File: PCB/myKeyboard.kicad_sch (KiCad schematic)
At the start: 6 parts, among them SW1 SW_Push, SW2 SW_Push, SW3 SW_Push, U1 XIAO-RP2040-DIP

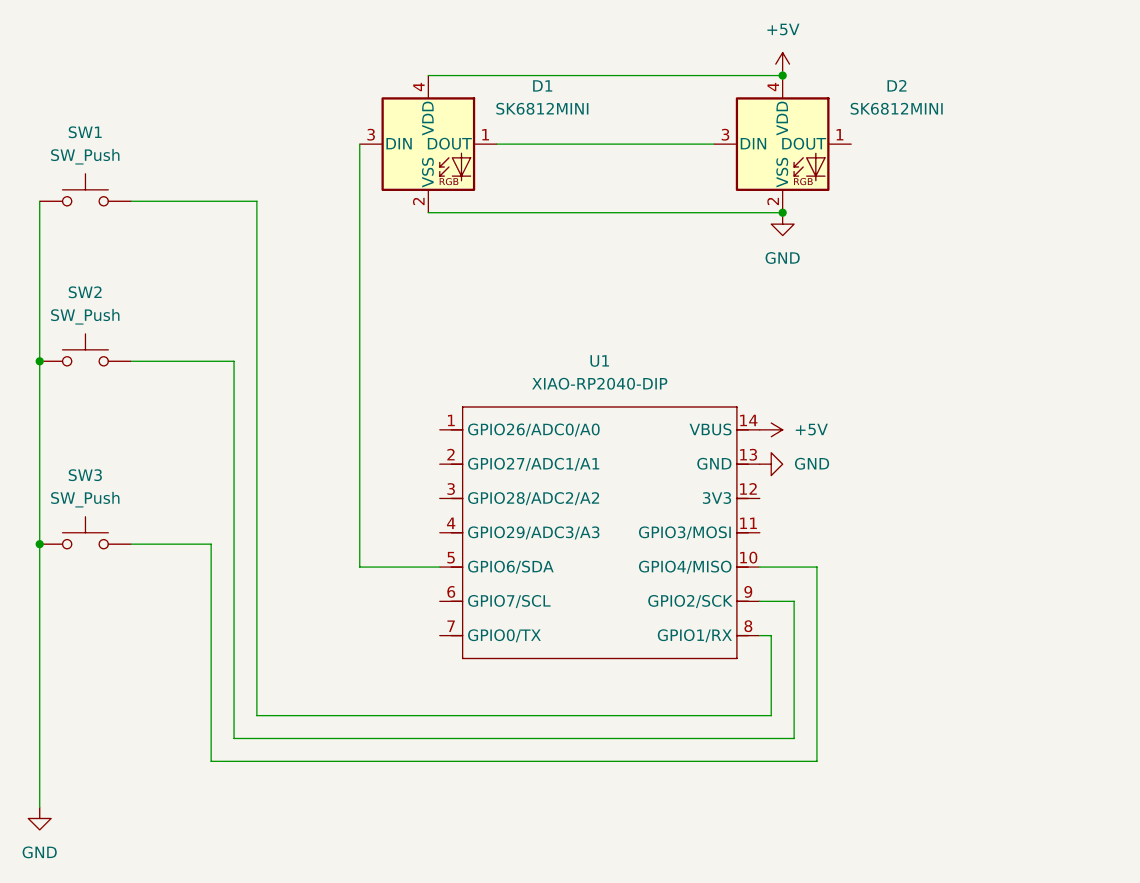
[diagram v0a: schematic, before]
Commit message: a
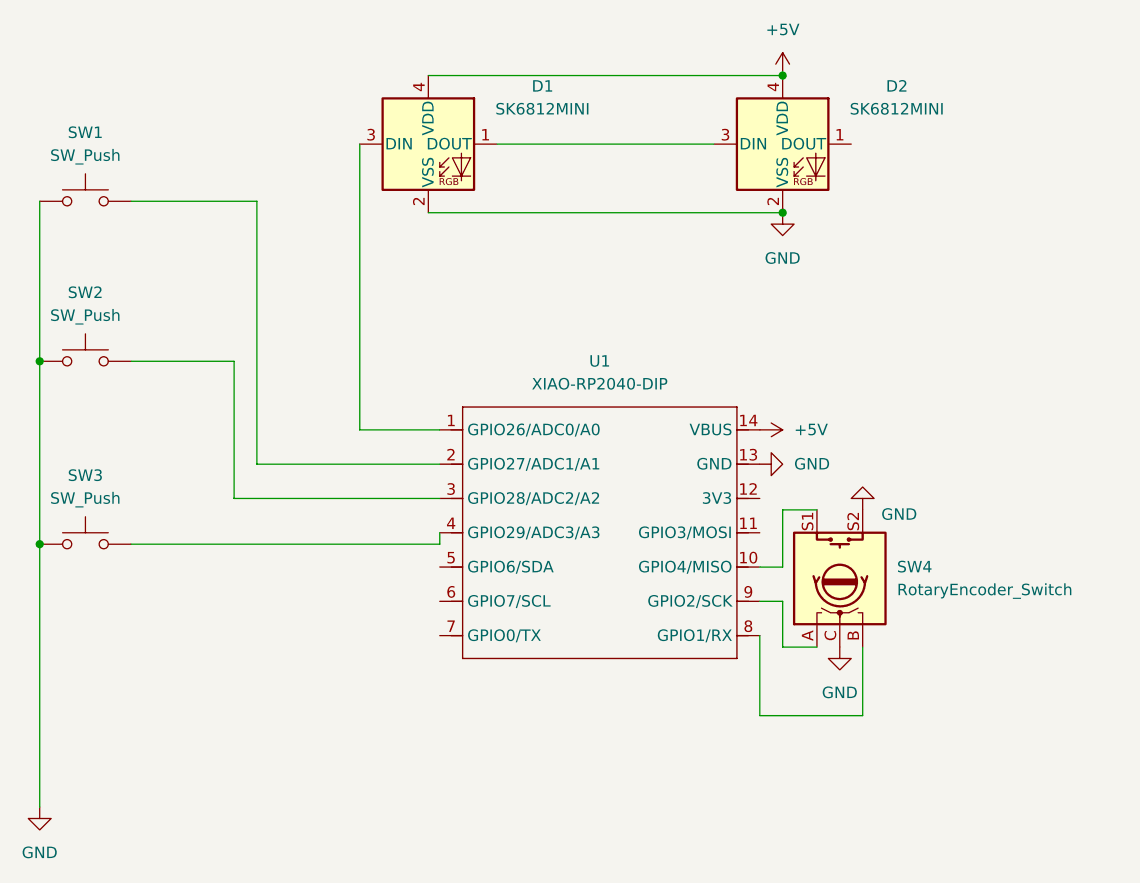
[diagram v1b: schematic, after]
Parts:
- added SW4: RotaryEncoder_Switch, Rotary_Encoder:RotaryEncoder_Alps_EC11E-Switch_Vertical_H20mm_MountingHoles, symbol Device:RotaryEncoder_Switch
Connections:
- net GND: now also SW4.C, SW4.S2
- net at SW1.2: now also U1.2 (GPIO27/ADC1/A1); no longer U1.8 (GPIO1/RX)
- net at SW2.2: now also U1.3 (GPIO28/ADC2/A2); no longer U1.9 (GPIO2/SCK)
- net at U1.10 (GPIO4/MISO): now also SW4.S1; no longer SW3.2
- net at D1.3 (DIN): now also U1.1 (GPIO26/ADC0/A0); no longer U1.5 (GPIO6/SDA)
- net at U1.4 (GPIO29/ADC3/A3): now also SW3.2
- new net: SW4.A, U1.9 (GPIO2/SCK)
- new net: SW4.B, U1.8 (GPIO1/RX)
